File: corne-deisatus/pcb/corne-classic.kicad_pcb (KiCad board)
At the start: 2 copper layers, 149.4 x 94.7 mm, 101 parts, among them J1 MJ-4PP-9, J2 OLED, J3 LED, P1 i2c-pin, P2 i2c-pin, SW1 SW_PUSH, SW10 SW_PUSH, SW11 SW_PUSH, SW12 SW_PUSH, SW13 SW_PUSH, SW14 SW_PUSH, SW15 SW_PUSH, SW16 SW_PUSH, SW17 SW_PUSH, SW18 SW_PUSH, SW19 SW_PUSH, SW2 SW_PUSH, SW20 SW_PUSH, SW21 SW_PUSH, SW22 SW_PUSH, SW3 SW_PUSH, SW4 SW_PUSH, SW5 SW_PUSH, SW6 SW_PUSH, SW7 SW_PUSH, SW8 SW_PUSH, SW9 SW_PUSH, U1 ProMicro

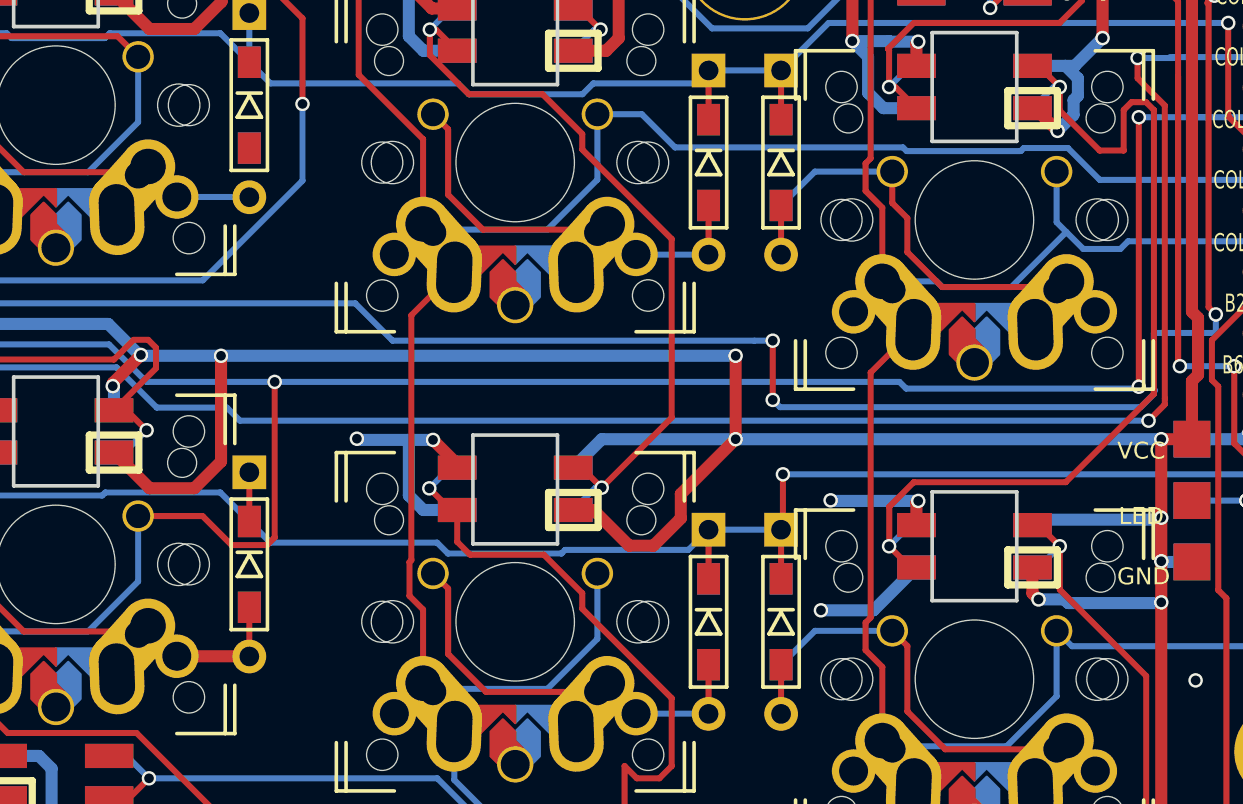
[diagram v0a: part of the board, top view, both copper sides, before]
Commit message: every thing connected
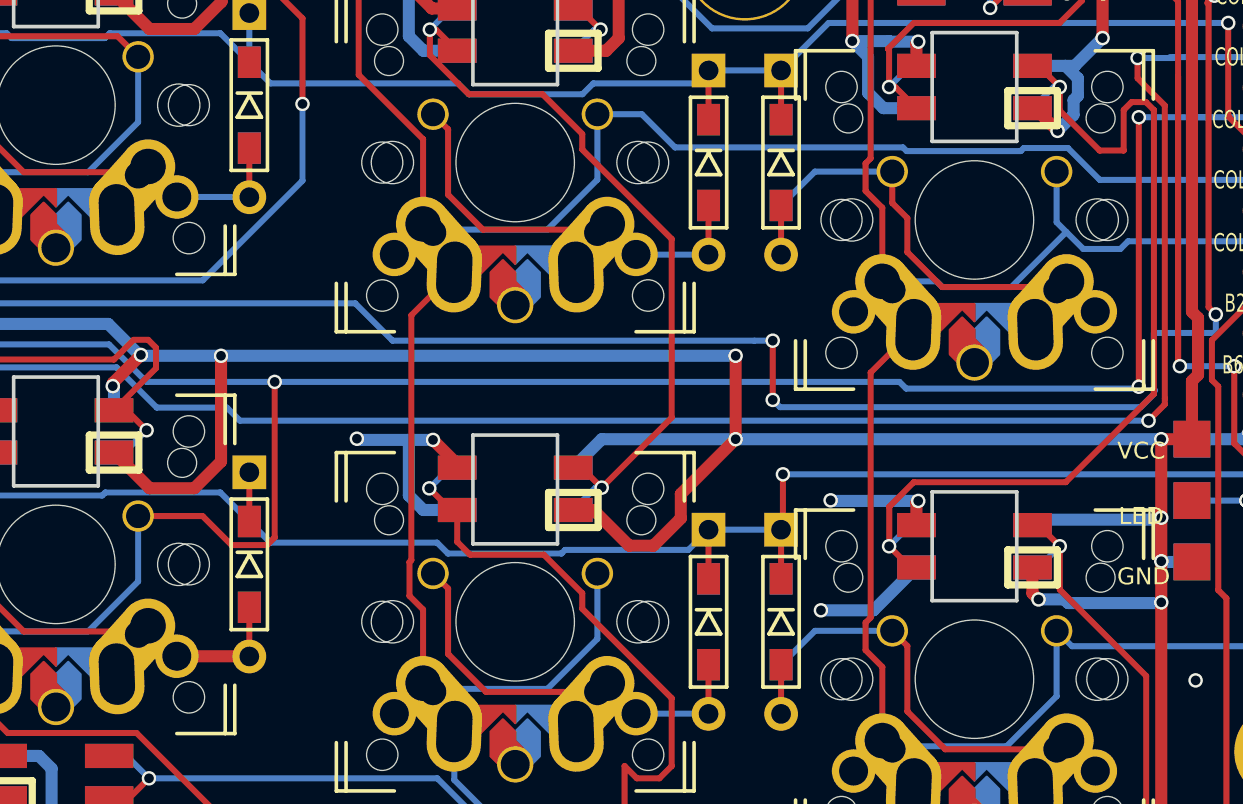
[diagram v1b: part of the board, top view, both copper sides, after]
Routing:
- net Net-(D10-Pad2): track 15.6 -> 17.7 mm
- net Net-(D12-Pad2): track 18.1 -> 19.8 mm
- net Net-(D16-Pad2): track 15.9 -> 17.7 mm
- net col5: track 195.5 -> 197.3 mm
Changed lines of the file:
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@@
     (thickness 1.6)
     (drawings 174)
-    (tracks 2440)
+    (tracks 2447)
     (zones 0)
     (modules 101)
@@
   (segment (start 130.81 91.61) (end 132 92.8) (width 0.25) (layer F.Cu) (net 14))
   (segment (start 130.81 91.54) (end 130.81 91.61) (width 0.25) (layer F.Cu) (net 14))
+  (segment (start 135 92.81) (end 135 90.775) (width 0.25) (layer F.Cu) (net 14))
   (segment (start 154 93.15) (end 154 95.185) (width 0.25) (layer F.Cu) (net 15))
   (segment (start 149.574999 94.150001) (end 149.81 93.915) (width 0.25) (layer F.Cu) (net 15))
@@
   (segment (start 158.4 91.75) (end 161.6 91.75) (width 0.25) (layer B.Cu) (net 16))
   (segment (start 157 93.15) (end 158.4 91.75) (width 0.25) (layer B.Cu) (net 16))
+  (segment (start 168.81 96.36) (end 170 97.55) (width 0.25) (layer F.Cu) (net 16))
+  (segment (start 168.81 96.29) (end 168.81 96.36) (width 0.25) (layer F.Cu) (net 16))
   (segment (start 62 116.9) (end 62 118.935) (width 0.25) (layer F.Cu) (net 17))
   (segment (start 73.574999 117.900001) (end 73.81 117.665) (width 0.25) (layer F.Cu) (net 17))
@@
   (segment (start 134.99 111.8) (end 135 111.81) (width 0.5) (layer F.Cu) (net 20))
   (segment (start 132 111.8) (end 134.99 111.8) (width 0.5) (layer F.Cu) (net 20))
+  (segment (start 132 111.73) (end 130.81 110.54) (width 0.25) (layer F.Cu) (net 20))
+  (segment (start 132 111.8) (end 132 111.73) (width 0.25) (layer F.Cu) (net 20))
   (segment (start 154 112.15) (end 154 114.185) (width 0.25) (layer F.Cu) (net 21))
   (segment (start 144.793162 113.275164) (end 149.400008 113.275164) (width 0.25) (layer F.Cu) (net 21))
@@
   (segment (start 160 78.48) (end 161.19 77.29) (width 0.25) (layer F.Cu) (net 33))
   (segment (start 160 78.55) (end 160 78.48) (width 0.25) (layer F.Cu) (net 33))
+  (segment (start 160 97.48) (end 161.19 96.29) (width 0.25) (layer F.Cu) (net 33))
+  (segment (start 160 97.55) (end 160 97.48) (width 0.25) (layer F.Cu) (net 33))
   (segment (start 178.525162 73.042) (end 176.86 73.042) (width 0.25) (layer B.Cu) (net 34))
   (segment (start 179.795162 71.772) (end 178.525162 73.042) (width 0.25) (layer B.Cu) (net 34))
